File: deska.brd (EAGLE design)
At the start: 53 x 83.8 mm, 11 parts

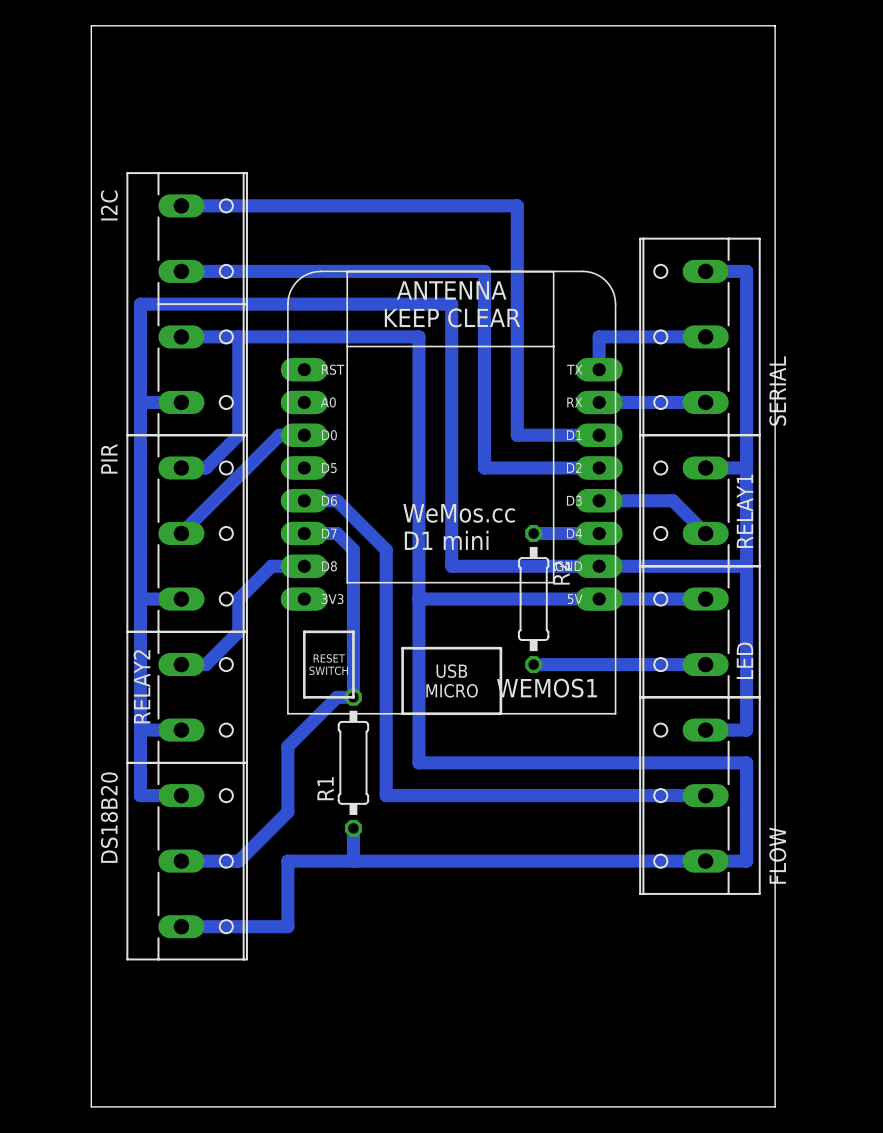
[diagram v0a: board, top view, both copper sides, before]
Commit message: board editing
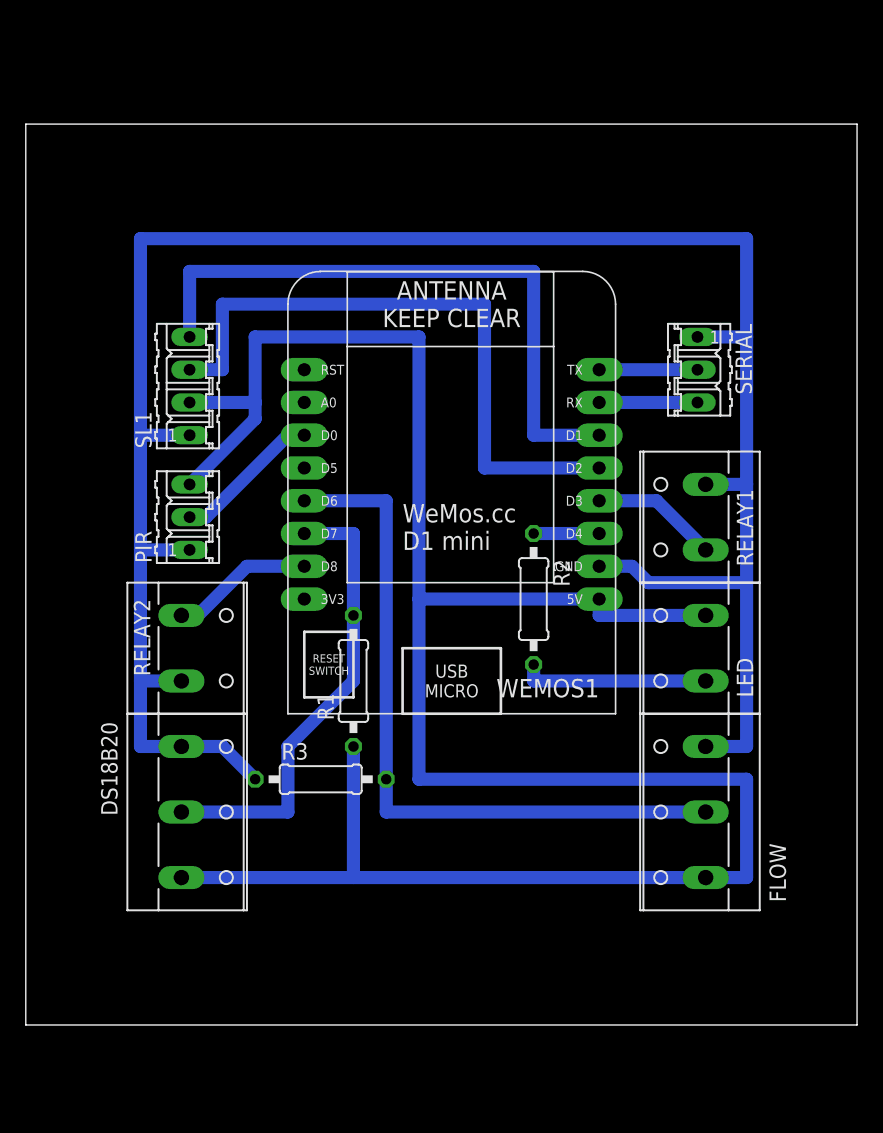
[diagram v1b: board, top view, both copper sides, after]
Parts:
- removed I2C: (no value), con-wago-508:W237-4P
- added R3: 220, rcl:0207/10
- added SL1: (no value), con-amp-quick:04P
- PIR, SERIAL: device con-wago-508:W237-133 -> con-amp-quick:03P
- moved R1 6.35 mm to (19.1, 19.1)
- moved DS18B20 3.81 mm to (6.35, 8.89)
- moved RELAY2 3.81 mm to (6.35, 21.6)
- moved SERIAL 2.54 mm to (45.7, 43.2), turned to 270 degrees
- moved RELAY1 1.27 mm to (45.7, 31.8)
- moved FLOW 1.27 mm to (45.7, 8.89)
- moved LED 1.27 mm to (45.7, 21.6)
- moved PIR 1.27 mm to (6.35, 31.8), turned to 90 degrees
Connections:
- net +5V: now also PIR.3, SL1.2; no longer I2C.3, PIR.1
- net GND: now also PIR.1, R3.1, SERIAL.1, SL1.1; no longer I2C.4, PIR.3, SERIAL.3
- net N$10: now also R3.2
- net N$2: now also SERIAL.3; no longer SERIAL.1
- net N$3: now also SL1.4; no longer I2C.1
- net N$4: now also SL1.3; no longer I2C.2
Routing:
- net GND: track 163.2 -> 168.6 mm
- net +5V: track 171.2 -> 176.1 mm
- net N$10: track 51.7 -> 55.2 mm
- net N$1: track 10.8 -> 7.62 mm
- net N$8: track 14.2 -> 11.1 mm
- net N$4: track 47.6 -> 49.5 mm
- net N$9: track 37.3 -> 35.8 mm
- net N$12: track 13.3 -> 14.6 mm
- net N$5: track 12.7 -> 11.5 mm
- net N$3: track 50.2 -> 49.5 mm
- net N$2: track 8.25 -> 7.62 mm
- net N$7: track 9.31 -> 9.83 mm
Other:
- board size 53 x 83.8 mm -> 64.4 x 69.8 mm
